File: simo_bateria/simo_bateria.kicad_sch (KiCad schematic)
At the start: 4 parts, among them J1 CONECTOR SALIDA, U2 cargador_bateria, U3 conversor_dc

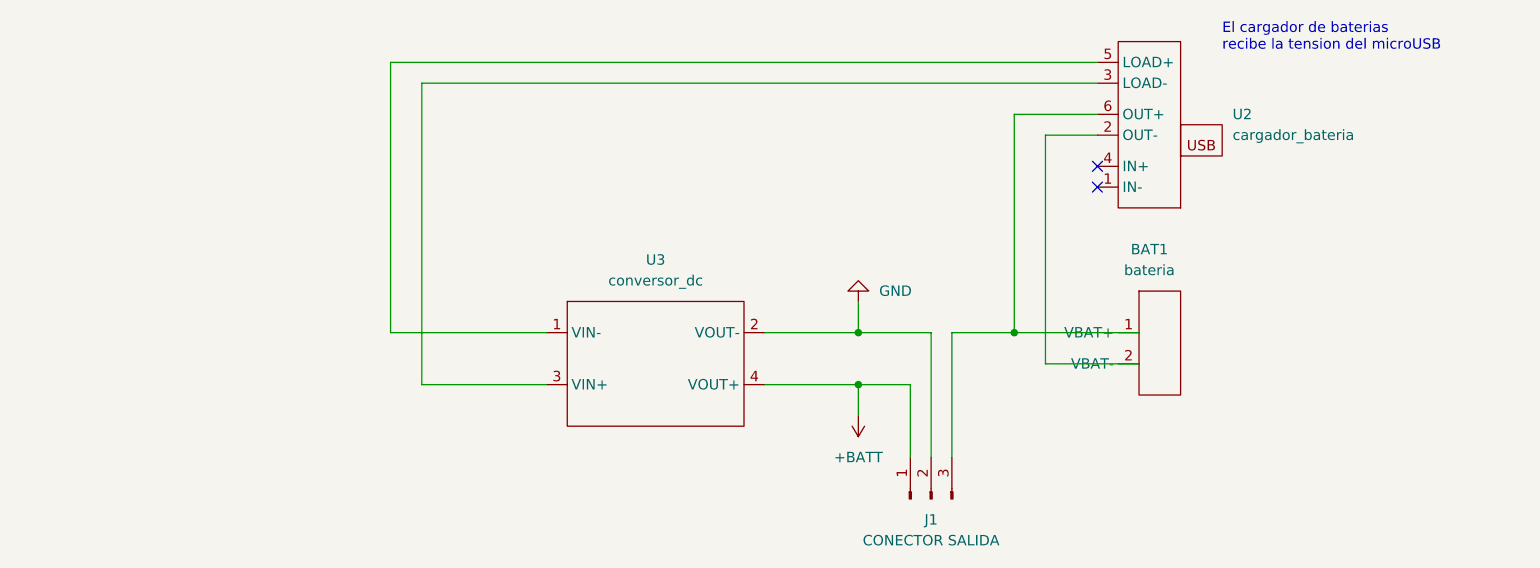
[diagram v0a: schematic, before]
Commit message: esquemas listos para revisar
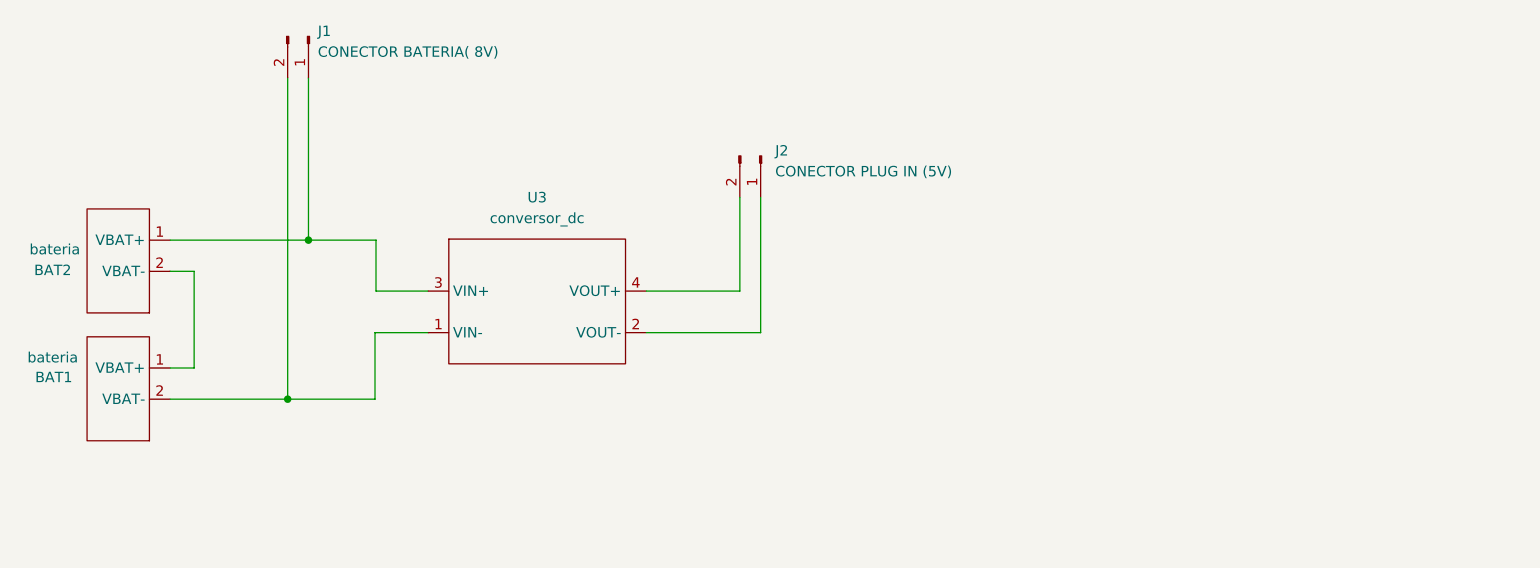
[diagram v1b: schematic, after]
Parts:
- removed J1: CONECTOR SALIDA, Connector_JST:JST_EH_B3B-EH-A_1x03_P2.50mm_Vertical, symbol Connector:Conn_01x03_Male
- removed U2: cargador_bateria, simo_bateria:cargador_bat, symbol simo_bateria:cargador_bateria
- added BAT2: bateria, Battery:BatteryHolder_MPD_BH-18650-PC2, symbol simo_bateria:bateria
- added J1: CONECTOR BATERIA( 8V), Connector_JST:JST_EH_B2B-EH-A_1x02_P2.50mm_Vertical, symbol Connector:Conn_01x02_Male
- added J2: CONECTOR PLUG IN (5V), Connector_JST:JST_EH_B2B-EH-A_1x02_P2.50mm_Vertical, symbol Connector:Conn_01x02_Male
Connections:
- net at BAT1.1 (VBAT+): now also BAT2.2 (VBAT-)
- net at BAT1.2 (VBAT-): now also U3.1 (VIN-), J1.2 (Pin_2)
- net at U3.3 (VIN+): now also BAT2.1 (VBAT+), J1.1 (Pin_1)
- net +BATT: no longer names the net of U3.4 (VOUT+)
- net +BATT: now also J2.2 (Pin_2)
- net GND: no longer names the net of U3.2 (VOUT-)
- net GND: now also J2.1 (Pin_1)
- no-connect marks 2 -> 0
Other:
- note removed: "El cargador de baterias recibe la tension del microUSB"
- moved on the sheet: U3
